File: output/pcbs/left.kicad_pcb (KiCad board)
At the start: 2 copper layers, 115 x 114 mm, 31 parts

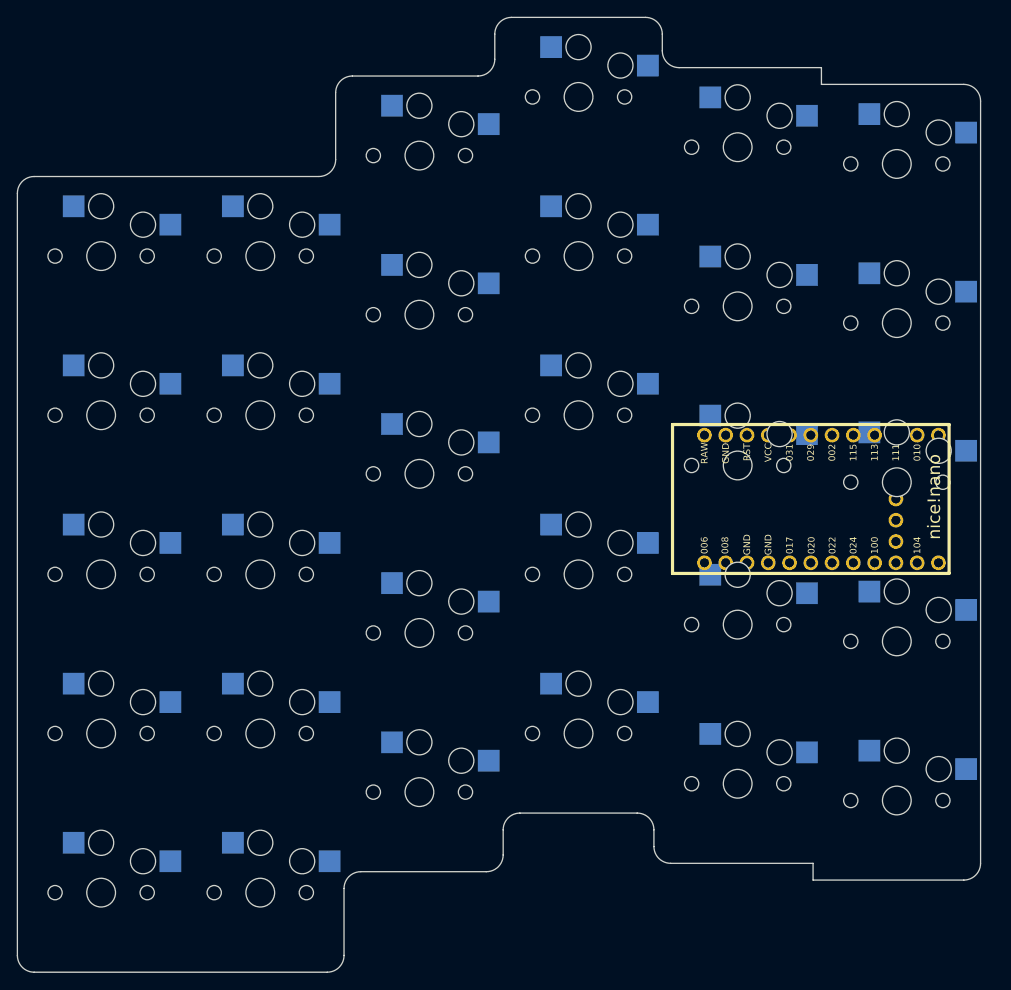
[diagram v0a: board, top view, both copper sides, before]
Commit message: sorry ilost track of time, just trying to fix the PCB
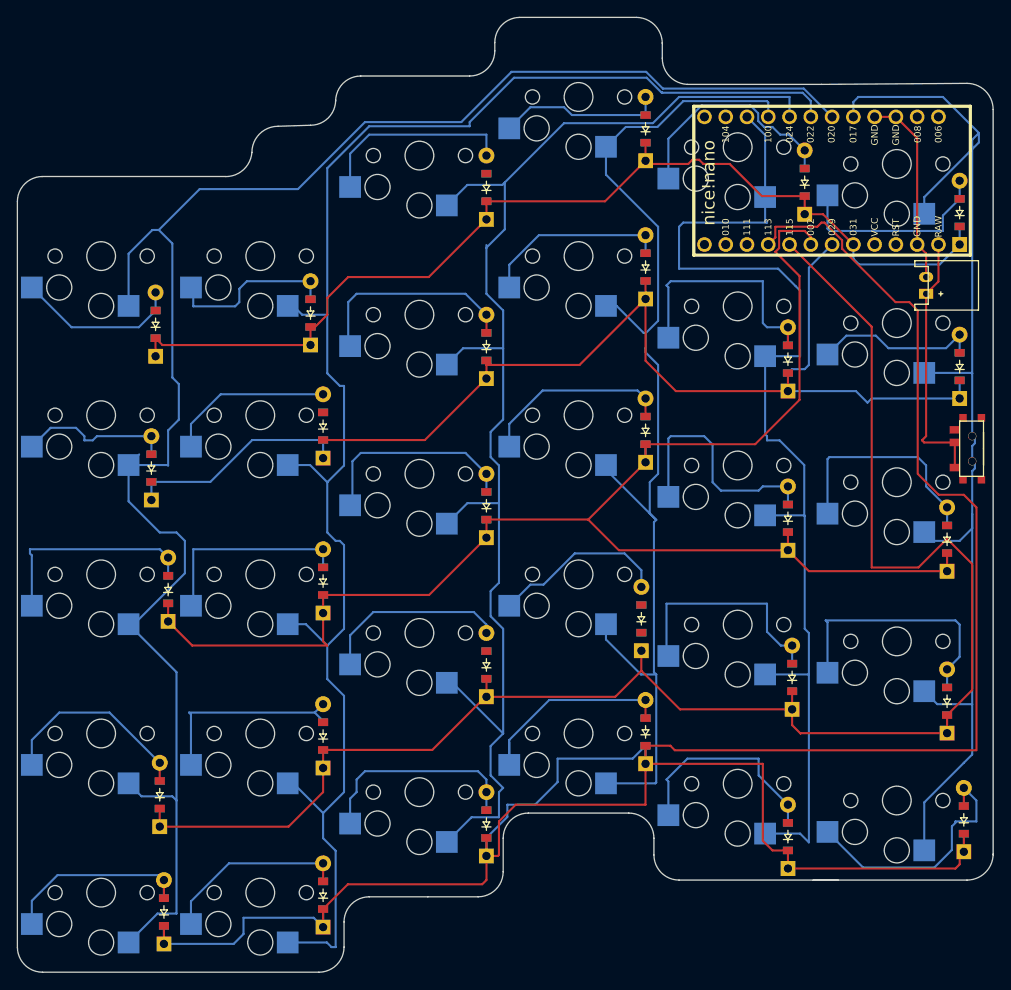
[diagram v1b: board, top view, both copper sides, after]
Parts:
- added D1: , ComboDiode, F.Cu at (7.50, 2.31)
- added D10: , ComboDiode, F.Cu at (25.0, -69.2)
- added D11: , ComboDiode, F.Cu at (46.0, -8.19)
- added D12: , ComboDiode, F.Cu at (46.0, -27.2)
- added D13: , ComboDiode, F.Cu at (46.0, -46.2)
- added D14: , ComboDiode, F.Cu at (46.0, -65.2)
- added D15: , ComboDiode, F.Cu at (46.0, -84.2)
- added D16: , ComboDiode, F.Cu at (65.0, -19.2)
- added D17: , ComboDiode, F.Cu at (64.5, -32.7)
- added D18: , ComboDiode, F.Cu at (65.0, -55.2)
- added D19: , ComboDiode, F.Cu at (65.0, -74.7)
- added D2: , ComboDiode, F.Cu at (7.00, -11.7)
- added D20: , ComboDiode, F.Cu at (65.0, -91.2)
- added D21: , ComboDiode, F.Cu at (82.0, -6.69)
- added D22: , ComboDiode, F.Cu at (82.5, -25.7)
- added D23: , ComboDiode, F.Cu at (82.0, -44.7)
- added D24: , ComboDiode, F.Cu at (82.0, -63.7)
- added D25: , ComboDiode, F.Cu at (84.0, -84.8)
- added D26: , ComboDiode, F.Cu at (103.0, -8.69)
- added D27: , ComboDiode, F.Cu at (101.0, -22.9)
- added D28: , ComboDiode, F.Cu at (101.0, -42.2)
- added D29: , ComboDiode, F.Cu at (102.5, -62.8)
- added D3: , ComboDiode, F.Cu at (8.00, -36.2)
- added D30: , ComboDiode, F.Cu at (102.5, -81.2)
- added D4: , ComboDiode, F.Cu at (6.00, -50.7)
- added D5: , ComboDiode, F.Cu at (6.50, -67.8)
- added D6: , ComboDiode, F.Cu at (26.5, 0.31)
- added D7: , ComboDiode, F.Cu at (26.5, -18.7)
- added D8: , ComboDiode, F.Cu at (26.5, -37.2)
- added D9: , ComboDiode, F.Cu at (26.5, -55.7)
- added JST1: , JST_PH_S2B-PH-K_02x2.00mm_Angled, F.Cu at (98.5, -72.5)
- added T1: , E73:SPDT_C128955, F.Cu at (104.0, -53.0)
- moved MCU1 38.0 mm to (86.0, -85.0), turned to 180 degrees
- turned S1 to 180 degrees
- turned S10 to 180 degrees
- turned S11 to 180 degrees
- turned S12 to 180 degrees
- turned S13 to 180 degrees
- turned S14 to 180 degrees
- turned S15 to 180 degrees
- turned S16 to 180 degrees
- turned S17 to 180 degrees
- turned S18 to 180 degrees
- turned S19 to 180 degrees
- turned S2 to 180 degrees
- turned S20 to 180 degrees
- turned S21 to 180 degrees
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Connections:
- S1 pad 2: P113 -> outer_num
- S10 pad 2: P031 -> pinky_mod
- S11 pad 2: P113 -> ring_num
- S12 pad 2: P115 -> ring_bottom
- S13 pad 2: P002 -> ring_home
- S14 pad 2: P029 -> ring_top
- S15 pad 2: P031 -> ring_mod
- S16 pad 2: P113 -> middle_num
- S17 pad 2: P115 -> middle_bottom
- S18 pad 2: P002 -> middle_home
- S19 pad 2: P029 -> middle_top
- S2 pad 2: P115 -> outer_bottom
- S20 pad 2: P031 -> middle_mod
- S21 pad 2: P113 -> index_num
- S22 pad 2: P115 -> index_bottom
- S23 pad 2: P002 -> index_home
- S24 pad 2: P029 -> index_top
- S25 pad 2: P031 -> index_mod
- S26 pad 2: P113 -> inner_num
- S27 pad 2: P115 -> inner_bottom
- S28 pad 2: P002 -> inner_home
- S29 pad 2: P029 -> inner_top
- S3 pad 2: P002 -> outer_home
- S30 pad 2: P031 -> inner_mod
- S4 pad 2: P029 -> outer_top
- S5 pad 2: P031 -> outer_mod
- S6 pad 2: P113 -> pinky_num
- S7 pad 2: P115 -> pinky_bottom
- S8 pad 2: P002 -> pinky_home
- S9 pad 2: P029 -> pinky_top
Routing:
- net P113: track 0.00 -> 293.1 mm
- net P020: track 0.00 -> 214.4 mm
- net P115: track 0.00 -> 196.5 mm
- net P022: track 0.00 -> 193.1 mm
- net P002: track 0.00 -> 176.0 mm
- net P024: track 0.00 -> 161.5 mm
- net P029: track 0.00 -> 145.9 mm
- net P017: track 0.00 -> 140.6 mm
- net P100: track 0.00 -> 134.9 mm
- net P011: track 0.00 -> 133.5 mm
- net P031: track 0.00 -> 124.4 mm
- net RAW: track 0.00 -> 31.2 mm
- net inner_bottom: track 0.00 -> 30.7 mm
- net index_top: track 0.00 -> 30.6 mm
- net inner_num: track 0.00 -> 30.3 mm
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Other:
- board size 115 x 114 mm -> 116.5 x 114 mm
- net class Default removed
